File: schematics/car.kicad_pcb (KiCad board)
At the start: 2 copper layers, 70.5 x 61.6 mm, 41 parts, among them IC1 ESP32-SOLO-1, J1 Conn_01x09_Female, J2 Conn_01x04_Male, J3 Conn_01x02_Female, J4 Conn_01x06_Female, J5 Conn_01x05_Female, J6 Conn_01x05_Female, M2.5 MountingHole_2.1mm, Q1 SS8050-G, Q2 SS8050-G, SW1 SW_Push, SW2 SW_Push, U1 L298HN

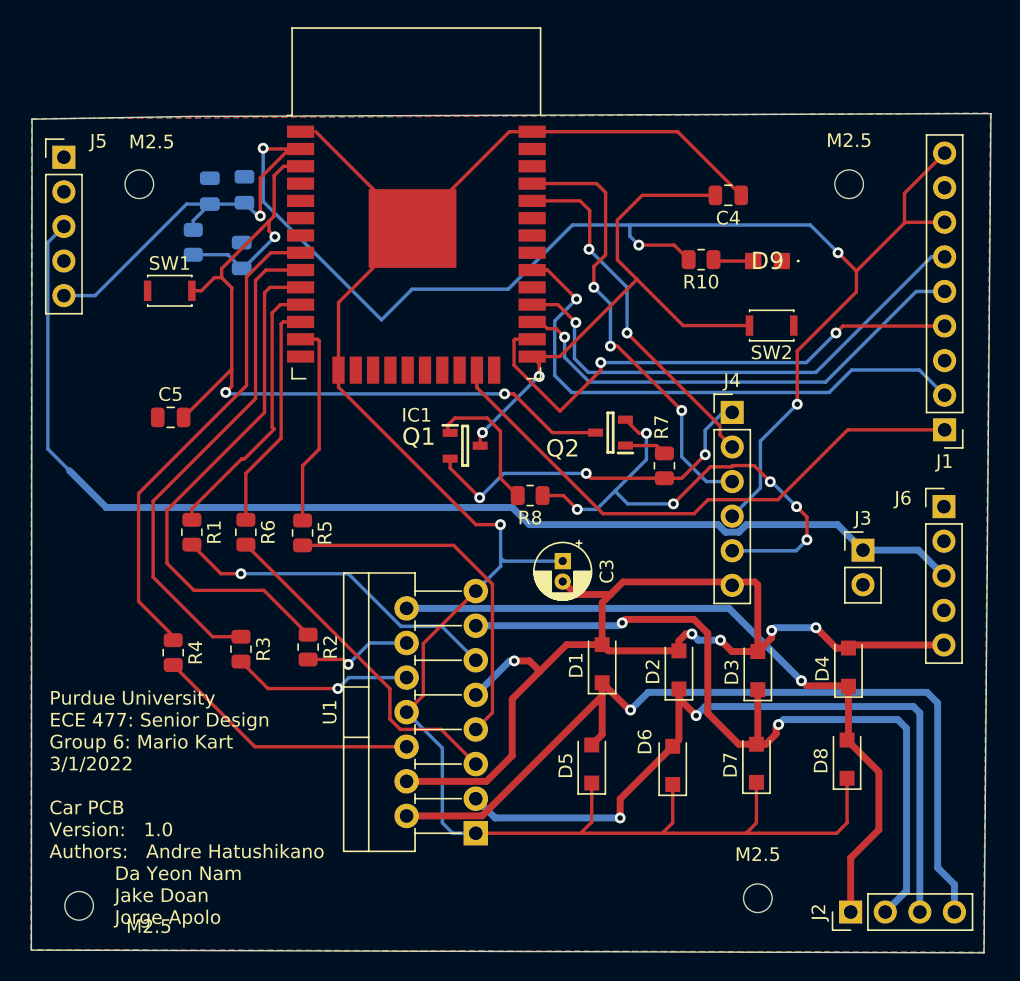
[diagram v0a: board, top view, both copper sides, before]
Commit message: final pcbs and schematics
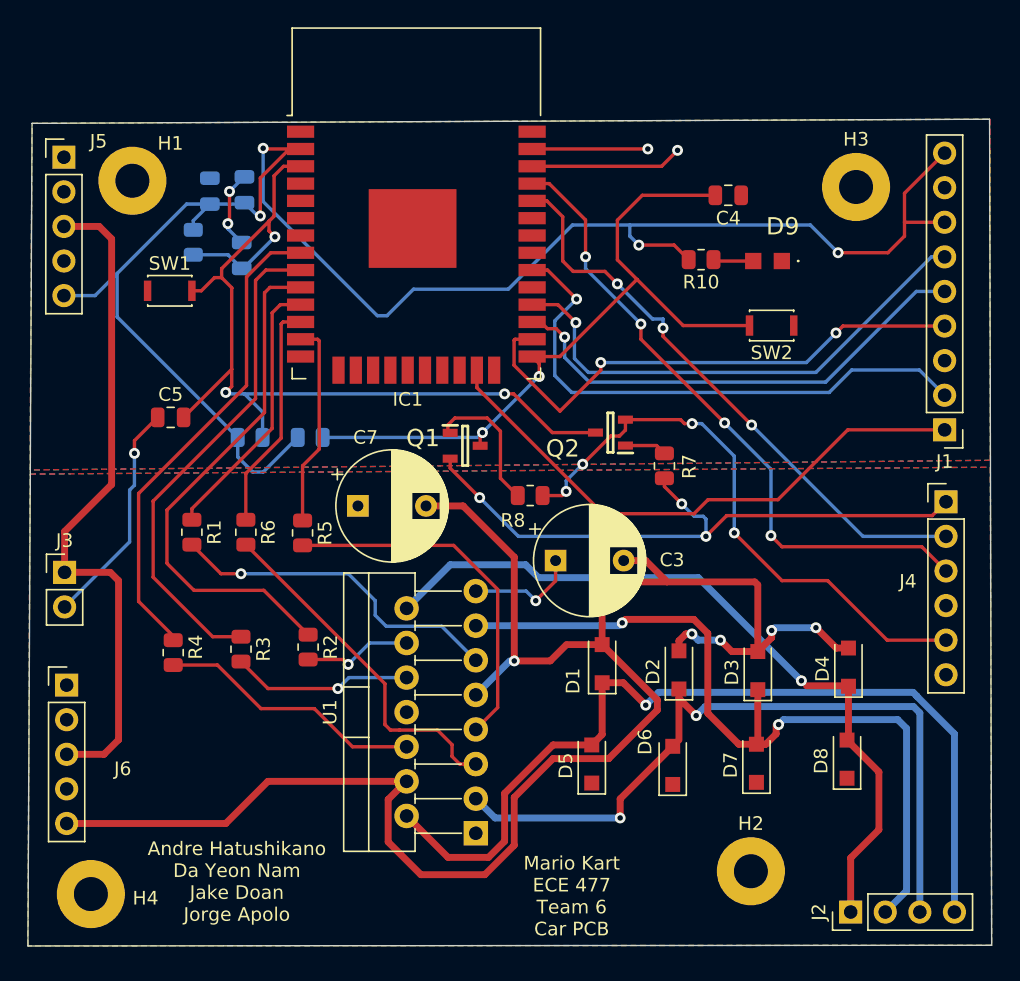
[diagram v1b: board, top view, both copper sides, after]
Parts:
- removed M2.5 (x4): MountingHole_2.1mm, MountingHole:MountingHole_2.1mm
- added C7: 100uF, Capacitor_THT:CP_Radial_D8.0mm_P5.00mm, F.Cu at (77.3, 78.8)
- added H1: MountingHole, MountingHole:MountingHole_2.5mm_Pad, F.Cu at (60.7, 54.9)
- added H2: MountingHole, MountingHole:MountingHole_2.5mm_Pad, F.Cu at (106.1, 105.6)
- added H3: MountingHole, MountingHole:MountingHole_2.5mm_Pad, F.Cu at (113.8, 55.4)
- added H4: MountingHole, MountingHole:MountingHole_2.5mm_Pad, F.Cu at (57.7, 107.3)
- added R11: 10k, Resistor_SMD:R_0805_2012Metric, B.Cu at (73.8, 73.8)
- added R12: 10k, Resistor_SMD:R_0805_2012Metric, B.Cu at (69.4, 73.8)
- C3: value 10uF -> 100uF; footprint Capacitor_THT:CP_Radial_D4.0mm_P1.50mm -> Capacitor_THT:CP_Radial_D8.0mm_P5.00mm
- moved J6 65.7 mm to (55.9, 91.9)
- moved J3 58.6 mm to (55.7, 83.7)
- moved J4 17.0 mm to (120.4, 78.5)
- moved C3 0.52 mm to (91.8, 82.8), turned to 0 degrees
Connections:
- IC1 pad 36: unconnected-(IC1-Pad36) -> GPIO22
- IC1 pad 37: unconnected-(IC1-Pad37) -> GPIO23
- J4 pad 4: 3.3V -> unconnected-(J4-Pad4)
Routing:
- net GND: track 145.1 -> 30.8 mm, vias 1 -> 4
- net Vout: track 79.5 -> 131.6 mm
- net B+: track 86.9 -> 50.0 mm
- net DTR: track 26.2 -> 46.1 mm
- net RX: track 26.1 -> 43.2 mm, vias 2 -> 3
- net TX: track 32.9 -> 47.8 mm, vias 3 -> 4
- net GPIO0: track 41.2 -> 53.1 mm
- net GPIO22: track 0.00 -> 11.2 mm, vias 0 -> 1
- net GPIO23: track 0.00 -> 8.50 mm, vias 0 -> 1
- net CTS: track 38.1 -> 42.8 mm, vias 6 -> 4
- net EN: track 64.9 -> 68.6 mm
- net OUT4: track 53.3 -> 55.9 mm
- net OUT1: track 65.1 -> 66.5 mm
- net Net-(R6-Pad2): track 24.9 -> 25.8 mm
- net Net-(R1-Pad2): track 24.4 -> 25.0 mm
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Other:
- board size 70.5 x 61.6 mm -> 70.8 x 60.7 mm
- board text added: "Andre Hatushikano Da Yeon Nam Jake Doan Jorge Apolo"
- board text added: "Mario Kart ECE 477 Team 6 Car PCB"
- board text removed: "Purdue University ECE 477: Senior Design Group 6: Mario Kart 3/1/2022 Car PCB Version: 1.0 Authors: Andre Hatushikano Da Yeon Nam Jake Doan Jorge Apolo"
